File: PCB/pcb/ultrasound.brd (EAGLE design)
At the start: 190 x 80 mm, 4 parts, among them J1 455-1750-1-ND, J2 455-1750-1-ND

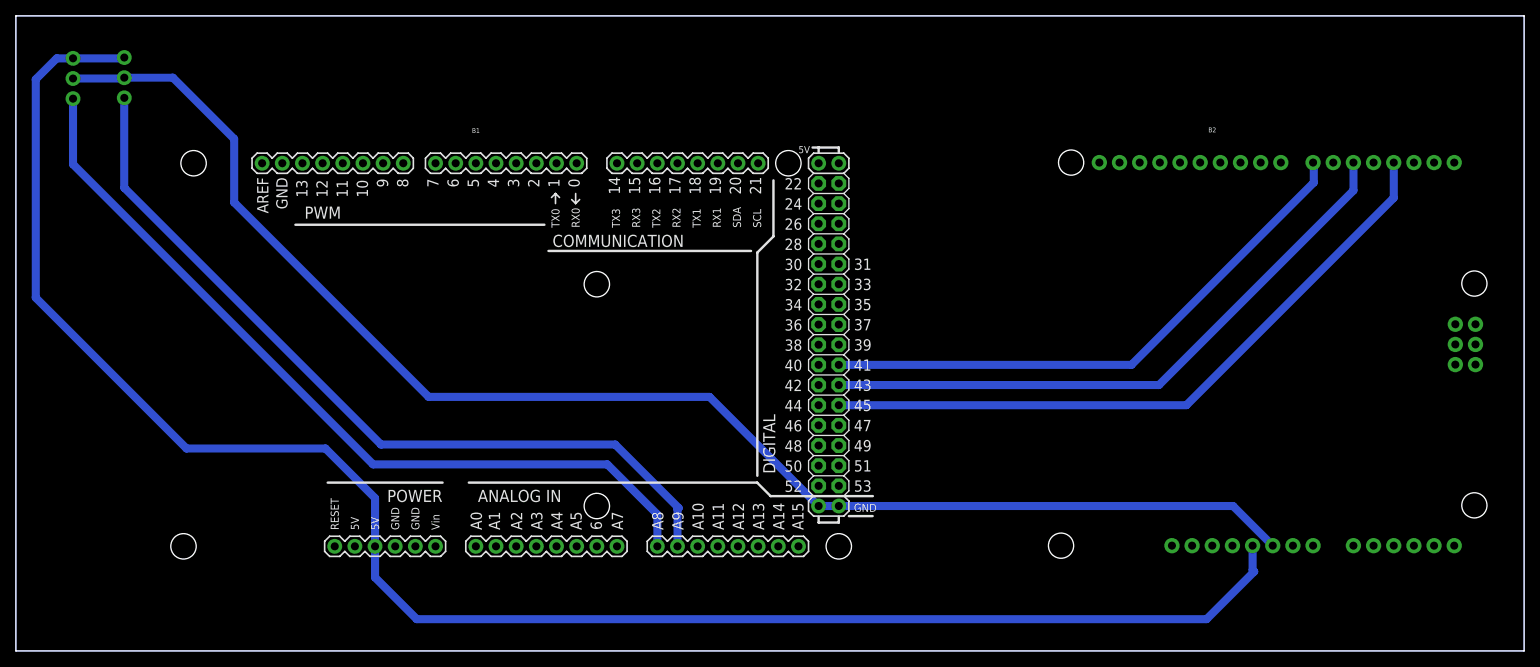
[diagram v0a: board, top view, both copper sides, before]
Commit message: pcb finale
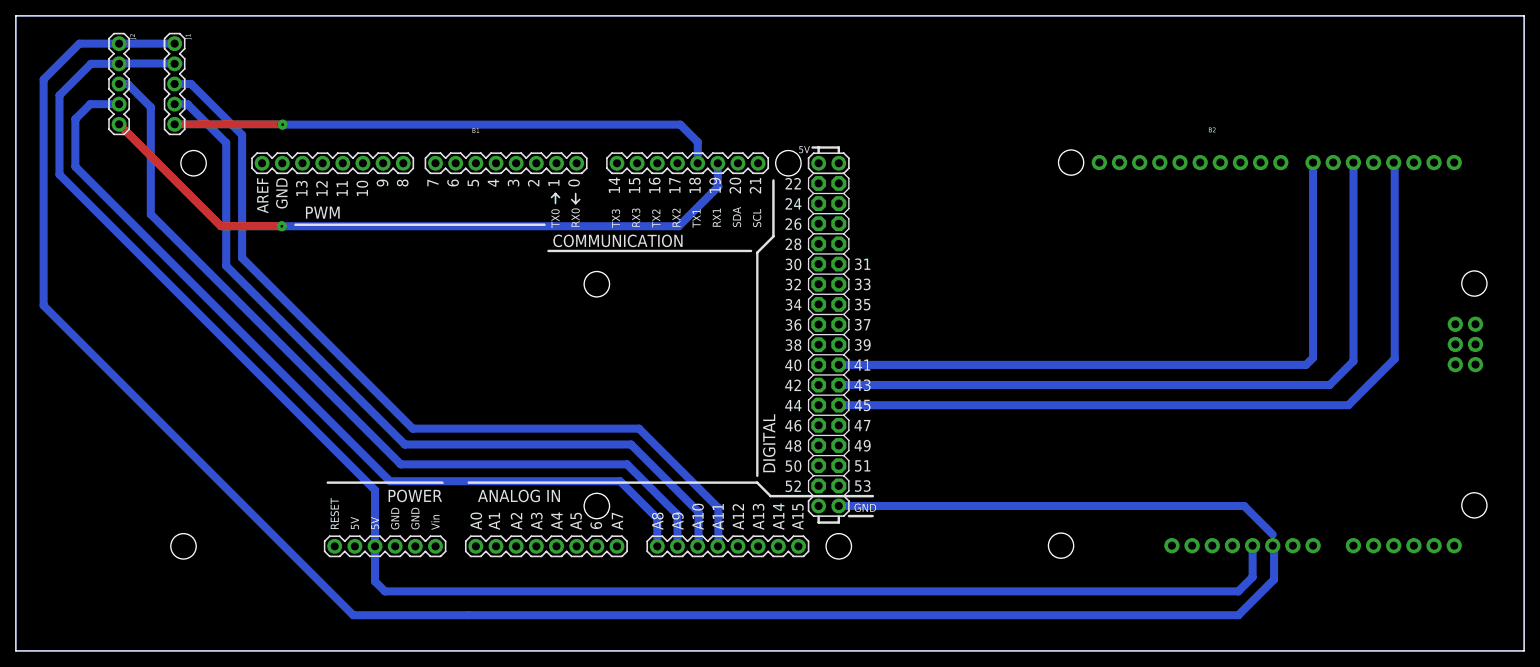
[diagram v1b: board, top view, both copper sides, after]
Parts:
- J1, J2: value 455-1750-1-ND -> (none); device SparkFun-Connectors:1X03 -> SparkFun-Connectors:1X05
- moved J1 14.6 mm to (100.0, 76.5), flipped to the top, turned to 270 degrees
- moved J2 6.86 mm to (93.0, 76.5), flipped to the top, turned to 270 degrees
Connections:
- removed net SHARP1: B1.A8, J1.1
- removed net SHARP2: B1.A9, J2.1
- new net GND2: B2.GND@1, J1.1, J2.1
- new net INT: B1.18, J1.5
- new net INT2: B1.19, J2.5
- new net SCL: B1.A10, J1.4
- new net SCL2: B1.A8, J2.4
- new net SDA: B1.A11, J1.3
- new net SDA2: B1.A9, J2.3
- net GND: no longer B1.GND@2, B2.GND@1, J1.2, J2.2
- net VCC: now also J1.2, J2.2; no longer J1.3, J2.3
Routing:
- net GND2: track 0.00 -> 224.2 mm
- net GND: track 180.3 -> 56.2 mm
- net SCL2: track 0.00 -> 107.5 mm
- net SDA2: track 0.00 -> 104.7 mm
- net SDA: track 0.00 -> 104.6 mm
- net SHARP1: track 104.2 -> 0.00 mm
- net SHARP2: track 102.8 -> 0.00 mm
- net SCL: track 0.00 -> 100.7 mm
- net INT2: track 0.00 -> 85.9 mm, vias 0 -> 1
- net INT: track 0.00 -> 69.5 mm, vias 0 -> 1
- net BLU: track 71.9 -> 84.7 mm
- net VERDE: track 78.5 -> 91.1 mm
- net ROSSO: track 85.2 -> 97.2 mm
- net VCC: track 221.8 -> 210.2 mm
